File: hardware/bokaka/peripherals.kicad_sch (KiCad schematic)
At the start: 7 parts, among them SW1 SW_MEC_5G, SW2 SW_MEC_5G, SW3 SW_MEC_5G, U3 IS31FL3236A-TQ

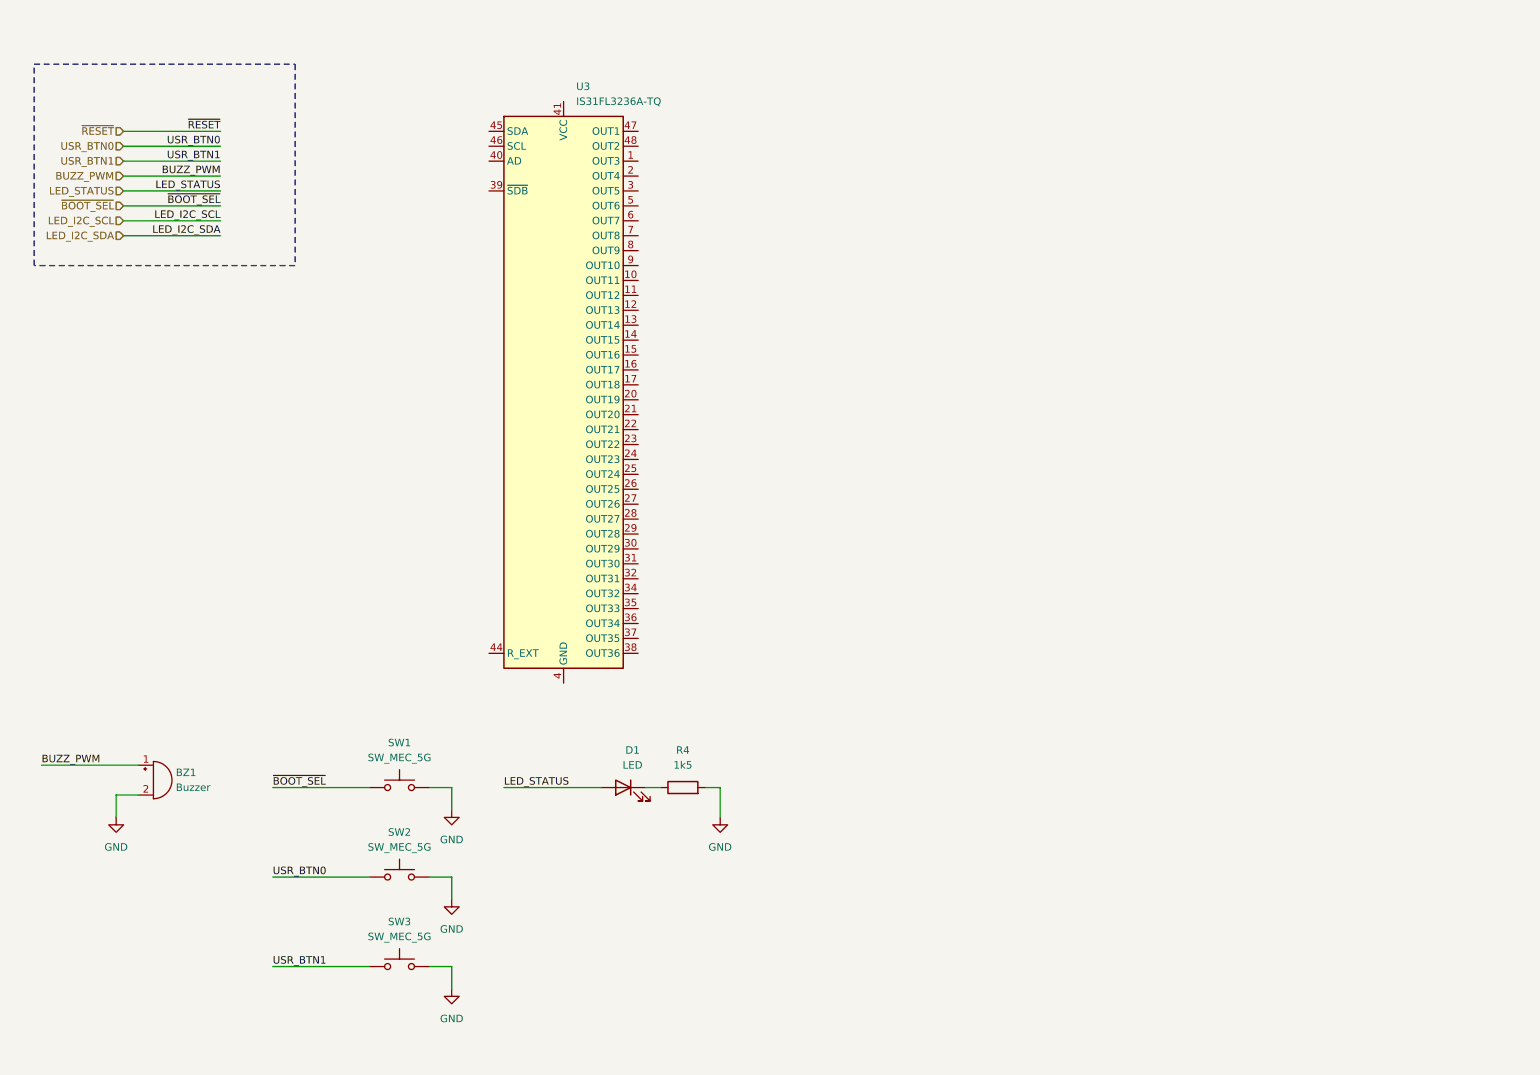
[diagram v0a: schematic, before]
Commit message: Finalize design before pcb
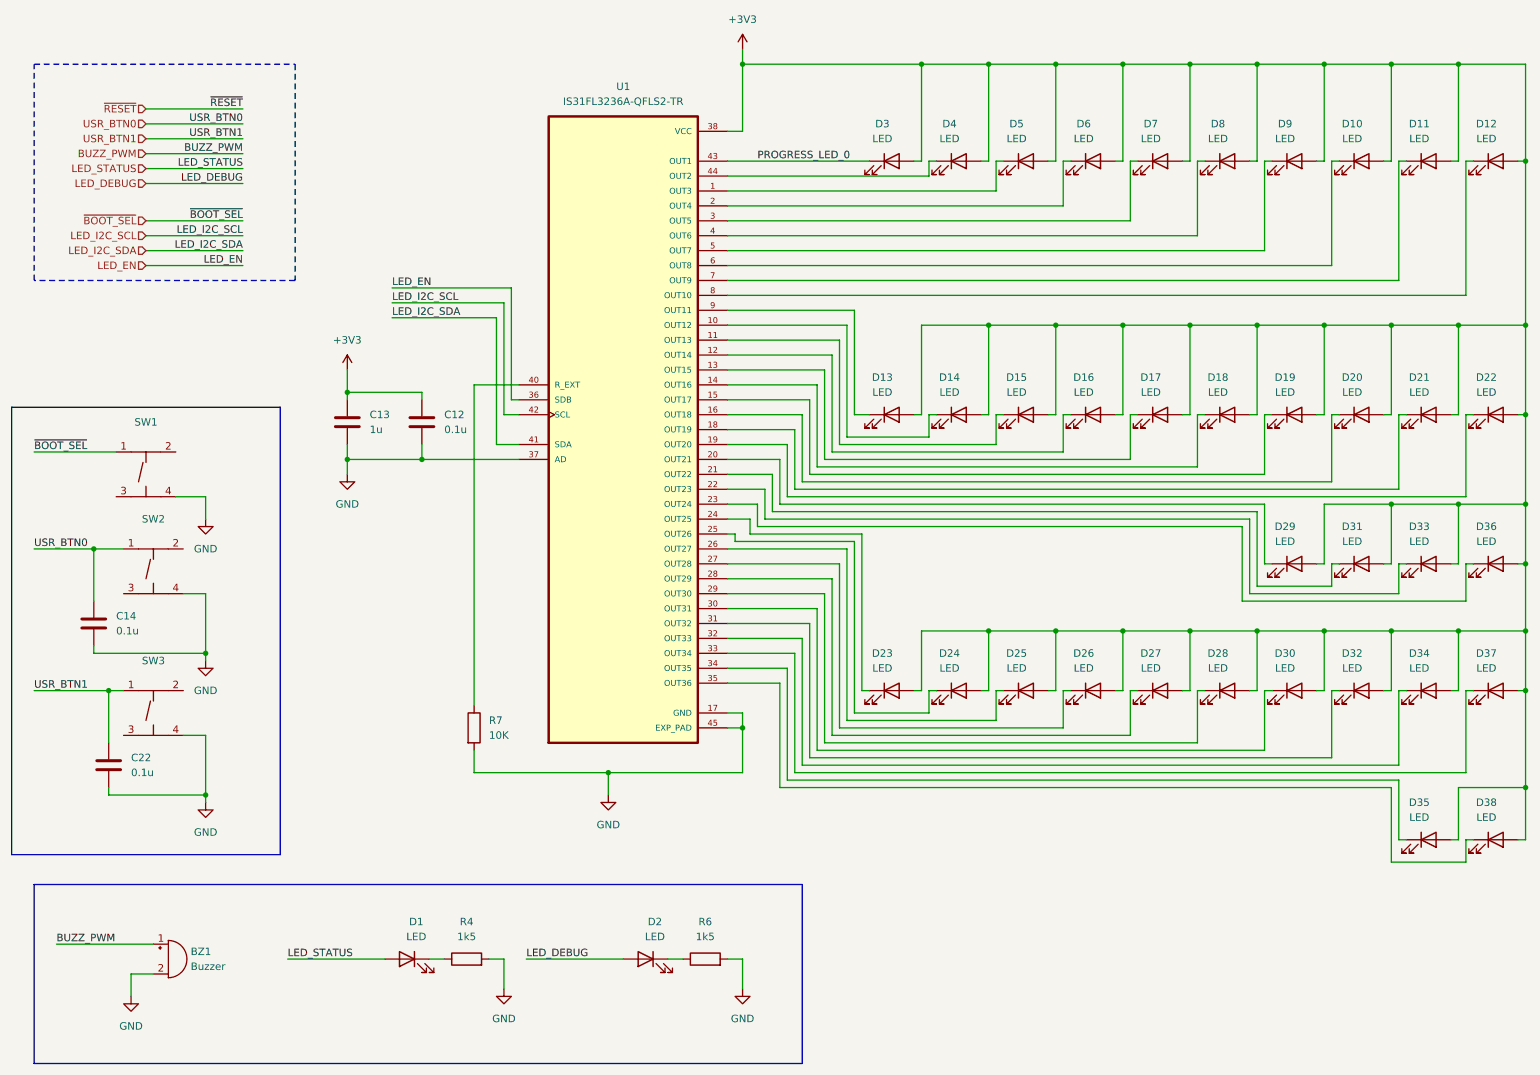
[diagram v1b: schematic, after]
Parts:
- removed SW1, SW2, SW3: SW_MEC_5G, symbol Switch:SW_MEC_5G
- removed U3: IS31FL3236A-TQ, Package_QFP:TQFP-48-1EP_7x7mm_P0.5mm_EP4.11x4.11mm, symbol Driver_LED:IS31FL3236A-TQ
- added C12, C14, C22: 0.1u, Capacitor_SMD:C_0402_1005Metric, symbol Device:C
- added C13: 1u, Capacitor_SMD:C_0402_1005Metric, symbol Device:C
- added D10, D11, D12, D13, D14, D15, D16, D17, D18, D19, D2, D20, D21, D22, D23, D24, D25, D26, D27, D28, D29, D3, D30, D31, D32, D33, D34, D35, D36, D37, D38, D4, D5, D6, D7, D8, D9: LED, symbol Device:LED
- added R6: 1k5, Resistor_SMD:R_0402_1005Metric, symbol Device:R
- added R7: 10K, Resistor_SMD:R_0402_1005Metric, symbol Device:R
- added SW1, SW2, SW3: ~, EasyEDA_Lib:SW-SMD_4P-L5.1-W5.1-P3.70-LS6.5-TL_H1.5, symbol EasyEDA_Lib:TS-1187A-B-A-B
- added U1: IS31FL3236A-QFLS2-TR, Footprints:QFN40P500X500X80-45N, symbol Symbols:IS31FL3236A-QFLS2-TR
- BZ1: footprint (none) -> Footprints:CUI_CPT-9019S-SMT
- R4: footprint (none) -> Resistor_SMD:R_0402_1005Metric
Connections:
- net GND: now also C12.2, C13.2, C14.2, C22.2, R6.2, R7.2, SW1.4 (D), SW2.4 (D), SW3.4 (D), U1.17 (GND), U1.37 (AD), U1.39 (GND), U1.45 (EXP_PAD)
- net LED_I2C_SCL: now also U1.42 (SCL)
- net LED_I2C_SDA: now also U1.41 (SDA)
- net USR_BTN0: now also C14.1, SW2.1 (A)
- net USR_BTN1: now also C22.1, SW3.1 (A)
- net ~{BOOT_SEL}: now also SW1.1 (A)
- new net: D5.1 (K), U1.1 (OUT3)
- new net: D27.1 (K), U1.28 (OUT29)
- new net: D17.1 (K), U1.13 (OUT15)
- new net: R7.1, U1.40 (R_EXT)
- new net: D18.1 (K), U1.14 (OUT16)
- new net: D25.1 (K), U1.26 (OUT27)
- new net: D14.1 (K), U1.10 (OUT12)
- new net: D15.1 (K), U1.11 (OUT13)
- new net: D13.1 (K), U1.9 (OUT11)
- new net: D2.1 (K), R6.1
- new net: D20.1 (K), U1.16 (OUT18)
- new net: D11.1 (K), U1.7 (OUT9)
- new net: D26.1 (K), U1.27 (OUT28)
- new net: D6.1 (K), U1.2 (OUT4)
- new net: D16.1 (K), U1.12 (OUT14)
- new net: D19.1 (K), U1.15 (OUT17)
- new net: D38.1 (K), U1.35 (OUT36)
- new net: D7.1 (K), U1.3 (OUT5)
- new net: D33.1 (K), U1.22 (OUT23)
- new net: D28.1 (K), U1.29 (OUT30)
- new net: D22.1 (K), U1.19 (OUT20)
- new net: D21.1 (K), U1.18 (OUT19)
- new net: D32.1 (K), U1.31 (OUT32)
- new net: D23.1 (K), U1.24 (OUT25)
- new net: D9.1 (K), U1.5 (OUT7)
- new net: D12.1 (K), U1.8 (OUT10)
- new net: D29.1 (K), U1.20 (OUT21)
- new net: D31.1 (K), U1.21 (OUT22)
- new net: D36.1 (K), U1.23 (OUT24)
- new net: D24.1 (K), U1.25 (OUT26)
- new net: D30.1 (K), U1.30 (OUT31)
- new net: D34.1 (K), U1.32 (OUT33)
- new net: D37.1 (K), U1.33 (OUT34)
- new net: D35.1 (K), U1.34 (OUT35)
- new net: D8.1 (K), U1.4 (OUT6)
- new net: D4.1 (K), U1.44 (OUT2)
- new net: D10.1 (K), U1.6 (OUT8)
- new net +3V3: C12.1, C13.1, D10.2 (A), D11.2 (A), D12.2 (A), D13.2 (A), D14.2 (A), D15.2 (A), D16.2 (A), D17.2 (A), D18.2 (A), D19.2 (A), D20.2 (A), D21.2 (A), D22.2 (A), D23.2 (A), D24.2 (A), D25.2 (A), D26.2 (A), D27.2 (A), D28.2 (A), D29.2 (A), D3.2 (A), D30.2 (A), D31.2 (A), D32.2 (A), D33.2 (A), D34.2 (A), D35.2 (A), D36.2 (A), D37.2 (A), D38.2 (A), D4.2 (A), D5.2 (A), D6.2 (A), D7.2 (A), D8.2 (A), D9.2 (A), U1.38 (VCC)
- new net LED_DEBUG: D2.2 (A)
- new net LED_EN: U1.36 (SDB)
- new net PROGRESS_LED_0: D3.1 (K), U1.43 (OUT1)
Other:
- moved on the sheet: BZ1, D1, R4
